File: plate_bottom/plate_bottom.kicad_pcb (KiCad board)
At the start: 2 copper layers, 179.7 x 122.7 mm, 24 parts, among them SW1 SW_Push, SW10 SW_Push, SW12 SW_Push, SW19 SW_Push, SW20 SW_Push, SW27 SW_Push, SW28 SW_Push, SW30 SW_Push, SW32 SW_Push, SW4 SW_Push, SW6 SW_Push, SW7 SW_Push

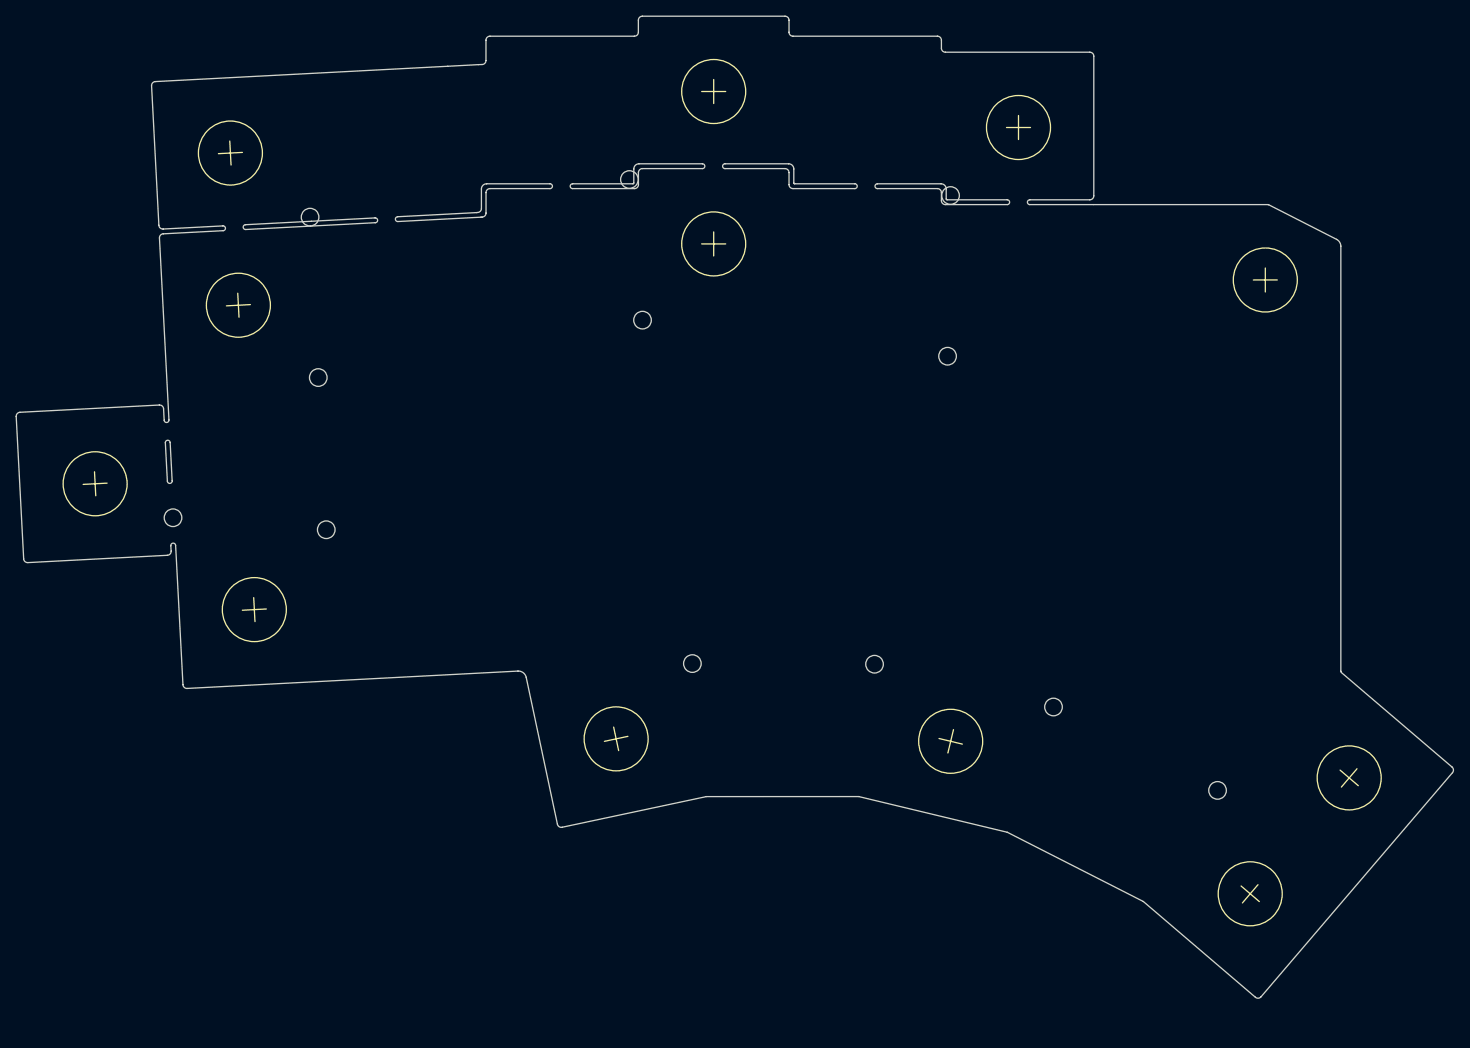
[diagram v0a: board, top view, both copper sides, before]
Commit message: Final changes of palm release.
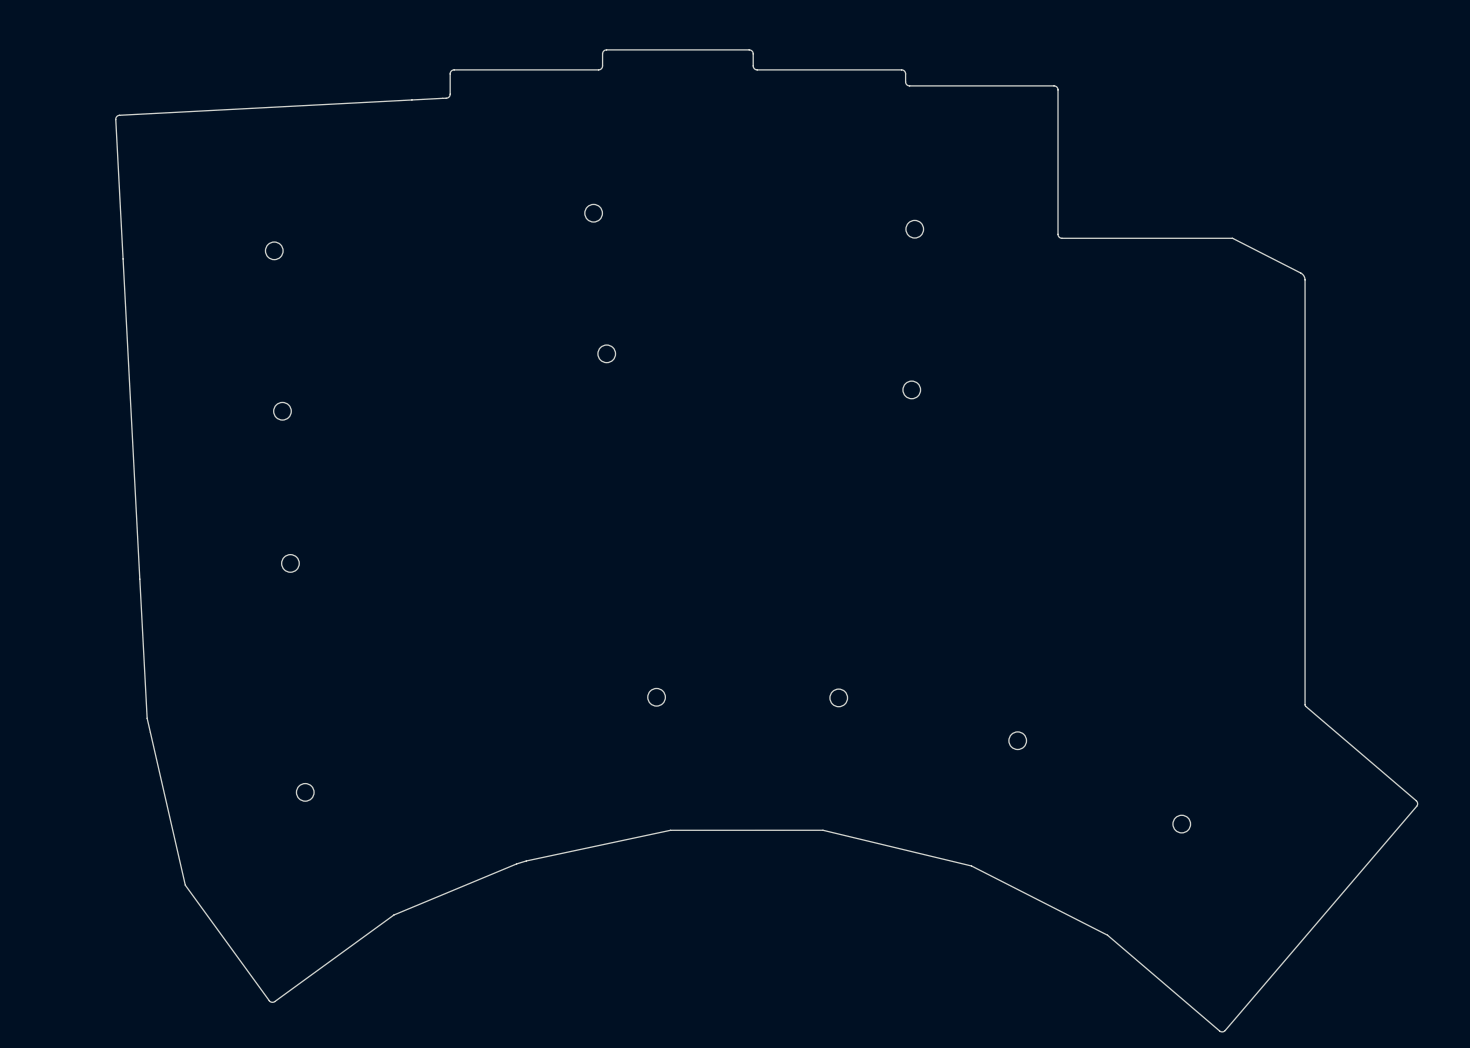
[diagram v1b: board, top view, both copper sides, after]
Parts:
- removed HM10, HM11, HM2, HM5, HM7, HM9: CaseHole, used_footprints:M2_HOLE_PCB
- removed the HM6 at (100.1, 89.6)
- removed the HM8 at (99.1, 70.6)
- removed SW1, SW10, SW12, SW19, SW20, SW27, SW28, SW30, SW32, SW4, SW6, SW7: SW_Push, used_footprints:bumpon_mark
- added HM6: CaseHole, used_footprints:M2_HOLE_PCB, F.Cu at (97.5, 122.4)
- added HM6: CaseHole, used_footprints:M2_HOLE_PCB, F.Cu at (95.6, 93.8)
- added HM8: CaseHole, used_footprints:M2_HOLE_PCB, F.Cu at (133.5, 50.0)
- added HM8: CaseHole, used_footprints:M2_HOLE_PCB, F.Cu at (173.3, 72.1)
- added HM8: CaseHole, used_footprints:M2_HOLE_PCB, F.Cu at (94.6, 74.8)
- added HM8: CaseHole, used_footprints:M2_HOLE_PCB, F.Cu at (135.1, 67.6)
- added HM8: CaseHole, used_footprints:M2_HOLE_PCB, F.Cu at (173.6, 52.0)
- added HM8: CaseHole, used_footprints:M2_HOLE_PCB, F.Cu at (93.6, 54.7)
- moved HM13 6.15 mm to (141.4, 110.6)
- moved HM3 6.15 mm to (207.0, 126.4)
- moved HM4 6.15 mm to (164.1, 110.6)
- moved HM14 6.15 mm to (186.5, 116.0)
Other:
- board size 179.7 x 122.7 mm -> 162.7 x 122.8 mm
- net class Default removed
